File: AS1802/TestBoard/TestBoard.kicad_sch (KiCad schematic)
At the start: 45 parts, among them J1 Screw_Terminal_01x02, J2 PORTA, J3 JTAG, J4 Conn_01x06, J5 PORTB, J6 SPI, SW1 SW_Push, U1 74LVC573, U2 IS62LV256AL, U3 EPM240T100, U4 W25Q32FVSS, U5 B2-CI2406, U6 MCP1319MT-29LE-OT, U7 AMS1117-1.8, U8 AMS1117-3.3, X1 CXO_DIP8

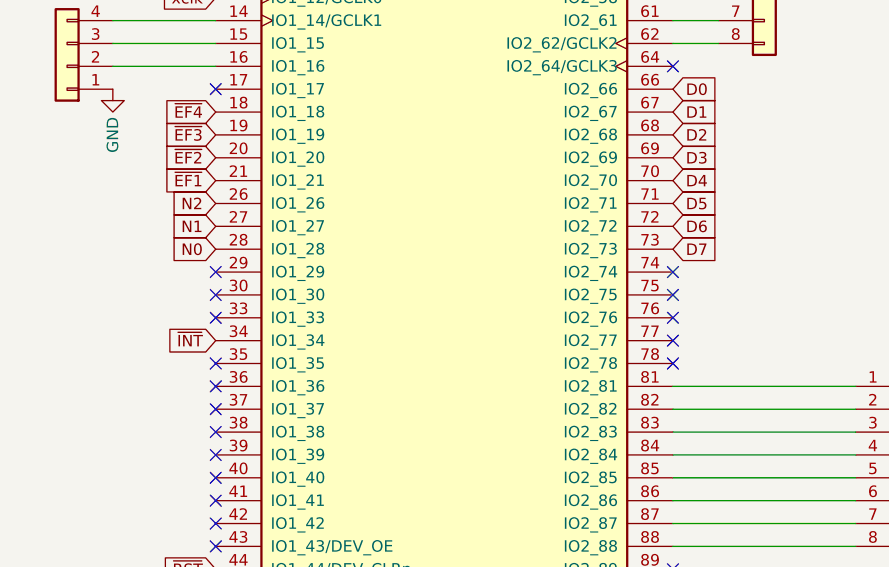
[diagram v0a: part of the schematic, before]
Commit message: VLIW ext4 progress
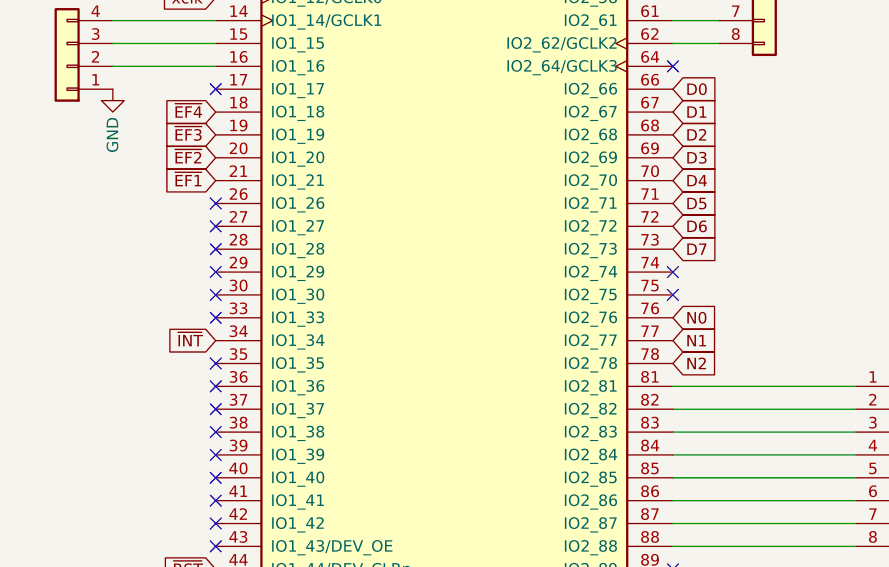
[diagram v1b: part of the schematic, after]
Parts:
- U2: footprint Package_SO:TSOP-I-28_11.8x8mm_P0.55mm -> TholinsStuff:TSOP-I-28_11.8x8mm_P0.55mm-weird-pin-order
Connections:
- net N0: now also U3.76 (IO2_76); no longer U3.28 (IO1_28)
- net N1: now also U3.77 (IO2_77); no longer U3.27 (IO1_27)
- net N2: now also U3.78 (IO2_78); no longer U3.26 (IO1_26)
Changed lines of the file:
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@@
 	)
 	(no_connect
+		(at 294.64 83.82)
+	)
+	(no_connect
 		(at 294.64 116.84)
 	)
@@
 	)
 	(no_connect
-		(at 345.44 99.06)
-	)
-	(no_connect
 		(at 41.91 100.33)
 	)
@@
 	)
 	(no_connect
+		(at 294.64 81.28)
+	)
+	(no_connect
 		(at 345.44 132.08)
 	)
@@
 	)
 	(no_connect
-		(at 345.44 96.52)
-	)
-	(no_connect
 		(at 345.44 66.04)
 	)
@@
 	)
 	(no_connect
-		(at 345.44 93.98)
+		(at 294.64 86.36)
 	)
 	(no_connect
@@
 		)
 	)
-	(global_label "N0"
-		(shape input)
-		(at 294.64 86.36 180)
-		(fields_autoplaced yes)
-		(effects
-			(font
-				(size 1.27 1.27)
-			)
-			(justify right)
-		)
-		(property "Intersheetrefs" "${INTERSHEET_REFS}"
-			(at 289.1148 86.36 0)
-			(effects
-				(font
-					(size 1.27 1.27)
-				)
-				(justify right)
-				(hide yes)
-			)
-		)
-	)
 	(global_label "CS29"
 		(shape input)
@@
 		)
 	)
-	(global_label "N1"
-		(shape input)
-		(at 294.64 83.82 180)
-		(fields_autoplaced yes)
-		(effects
-			(font
-				(size 1.27 1.27)
-			)
-			(justify right)
-		)
-		(property "Intersheetrefs" "${INTERSHEET_REFS}"
-			(at 289.1148 83.82 0)
-			(effects
-				(font
-					(size 1.27 1.27)
-				)
-				(justify right)
-				(hide yes)
-			)
-		)
-	)
 	(global_label "A6"
 		(shape input)
@@
 		)
 	)
+	(global_label "N2"
+		(shape input)
+		(at 345.44 99.06 0)
+		(fields_autoplaced yes)
+		(effects
+			(font
+				(size 1.27 1.27)
+			)
+			(justify left)
+		)
+		(property "Intersheetrefs" "${INTERSHEET_REFS}"
+			(at 350.9652 99.06 0)
+			(effects
+				(font
+					(size 1.27 1.27)
+				)
+				(justify left)
+				(hide yes)
+			)
+		)
+	)
 	(global_label "A2"
 		(shape input)
@@
 		)
 	)
+	(global_label "N1"
+		(shape input)
+		(at 345.44 96.52 0)
+		(fields_autoplaced yes)
+		(effects
+			(font
+				(size 1.27 1.27)
+			)
+			(justify left)
+		)
+		(property "Intersheetrefs" "${INTERSHEET_REFS}"
+			(at 350.9652 96.52 0)
+			(effects
+				(font
+					(size 1.27 1.27)
+				)
+				(justify left)
+				(hide yes)
+			)
+		)
+	)
 	(global_label "A2"
 		(shape input)
@@
 		)
 	)
-	(global_label "N2"
-		(shape input)
-		(at 294.64 81.28 180)
-		(fields_autoplaced yes)
-		(effects
-			(font
-				(size 1.27 1.27)
-			)
-			(justify right)
-		)
-		(property "Intersheetrefs" "${INTERSHEET_REFS}"
-			(at 289.1148 81.28 0)
-			(effects
-				(font
-					(size 1.27 1.27)
-				)
-				(justify right)
-				(hide yes)
-			)
-		)
-	)
 	(global_label "Q"
 		(shape input)
@@
 		)
 	)
+	(global_label "N0"
+		(shape input)
+		(at 345.44 93.98 0)
+		(fields_autoplaced yes)
+		(effects
+			(font
+				(size 1.27 1.27)
+			)
+			(justify left)
+		)
+		(property "Intersheetrefs" "${INTERSHEET_REFS}"
+			(at 350.9652 93.98 0)
+			(effects
+				(font
+					(size 1.27 1.27)
+				)
+				(justify left)
+				(hide yes)
+			)
+		)
+	)
 	(global_label "D7"
 		(shape input)
@@
 			)
 		)
-		(property "Footprint" "Package_SO:TSOP-I-28_11.8x8mm_P0.55mm"
+		(property "Footprint" "TholinsStuff:TSOP-I-28_11.8x8mm_P0.55mm-weird-pin-order"
 			(at 360.68 173.99 0)
 			(effects
